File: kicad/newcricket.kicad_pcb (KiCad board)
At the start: 2 copper layers, 32.5 x 49 mm, 25 parts, among them IC1 ATTINY85-P, Q1 Q_NPN_BCE, SW1 SW_PUSH, SW2 SW_PUSH, SW3 SWITCH_INV, U1 LM335

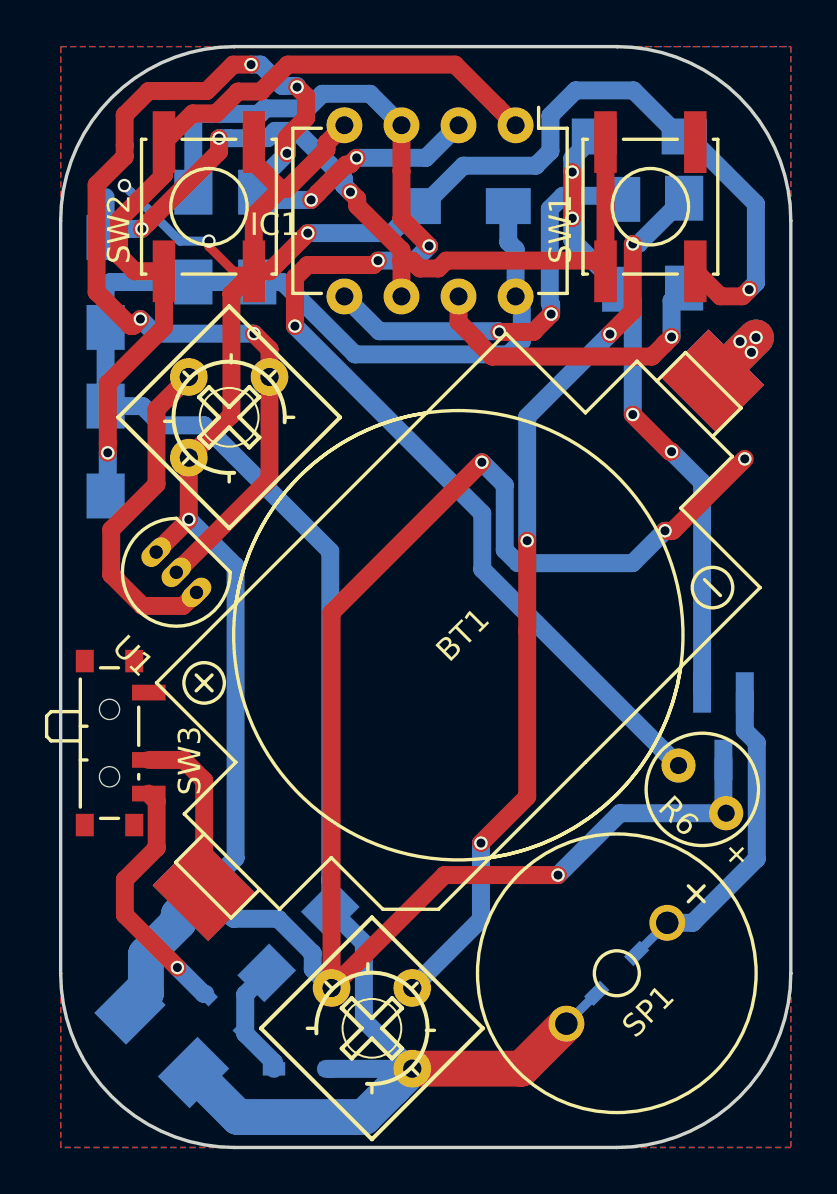
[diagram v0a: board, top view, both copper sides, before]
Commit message: removed old gerbers.
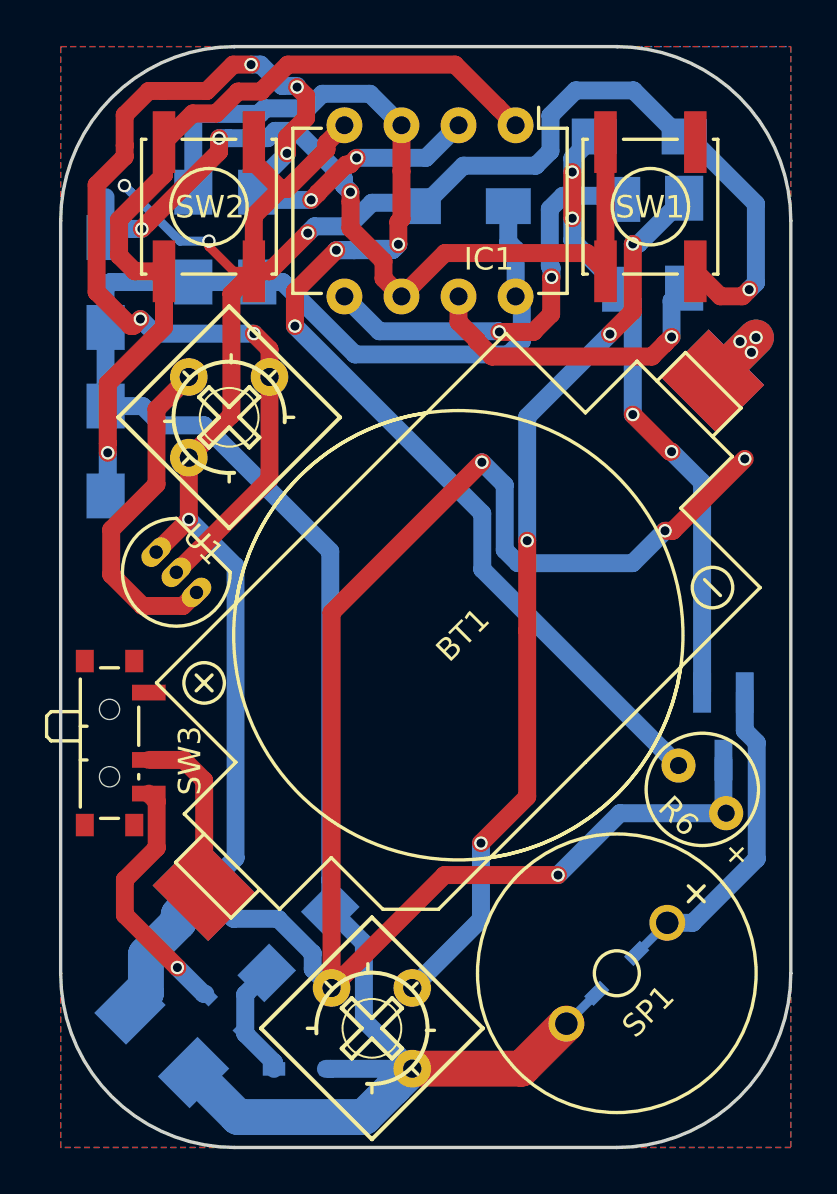
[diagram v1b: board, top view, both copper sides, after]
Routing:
- net Net-(IC1-Pad3): track 55.4 -> 56.1 mm
- net Net-(IC1-Pad6): track 37.2 -> 37.9 mm
